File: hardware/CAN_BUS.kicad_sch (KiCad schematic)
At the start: 15 parts, among them U7 ADM3057ExRW

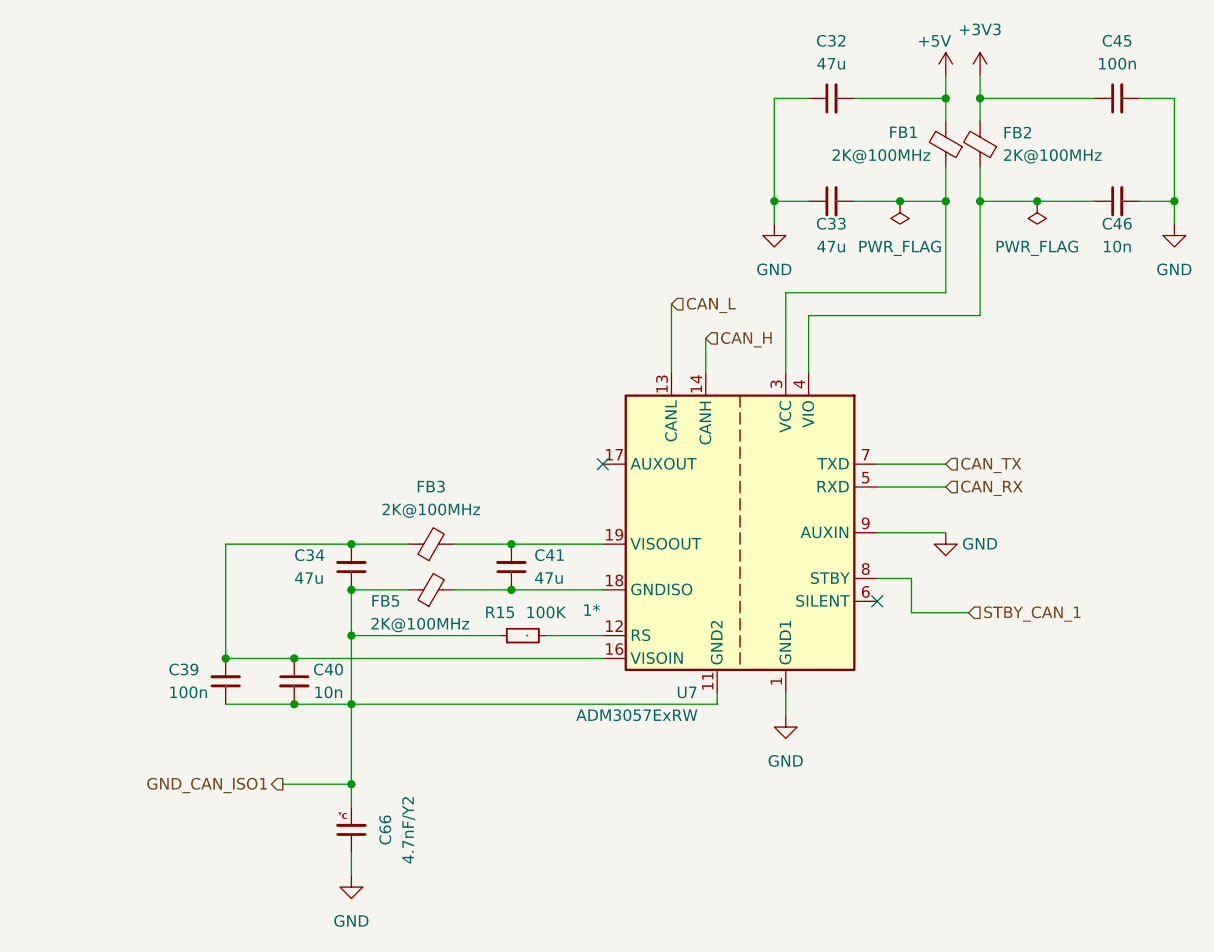
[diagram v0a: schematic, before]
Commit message: added missing files
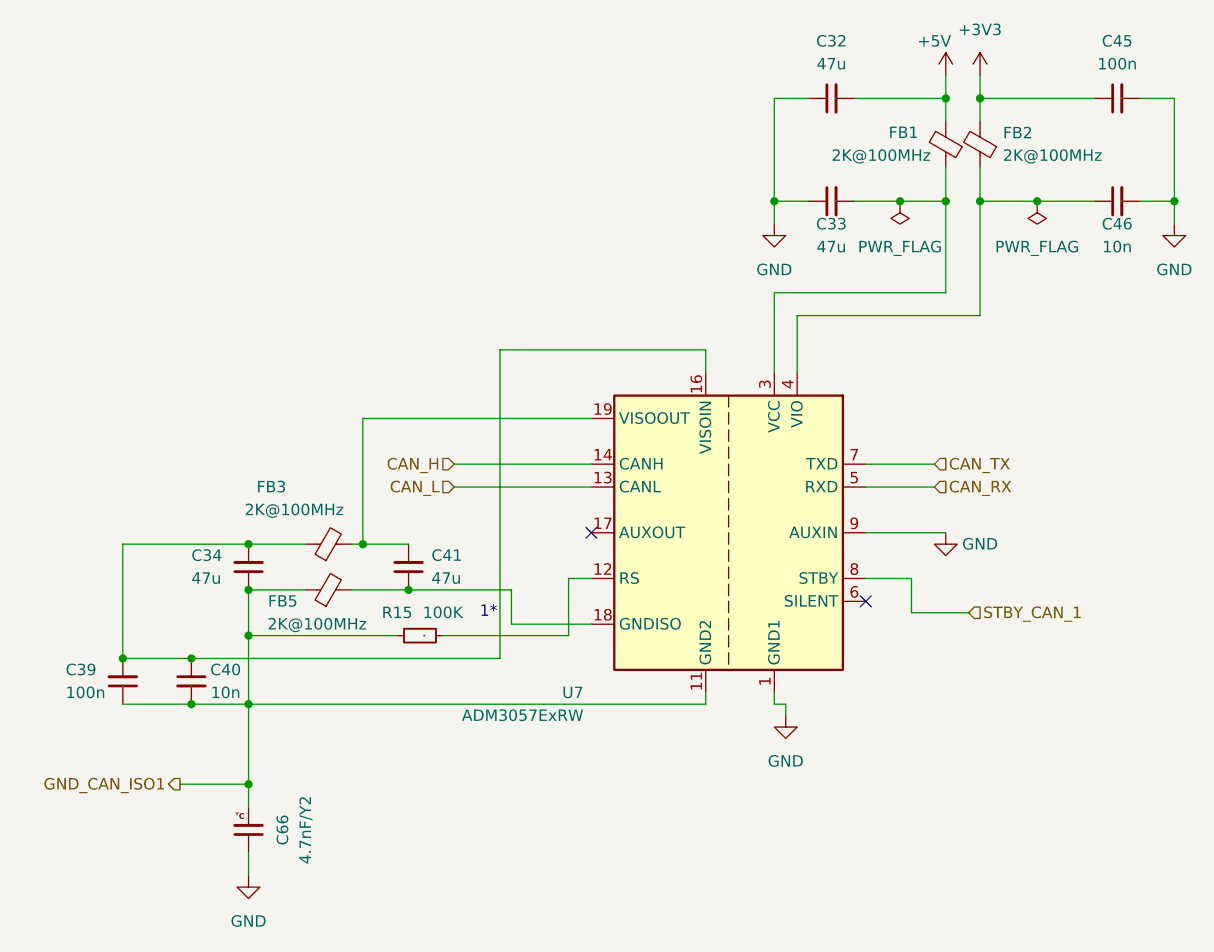
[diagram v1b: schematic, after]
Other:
- moved on the sheet: C34, C39, C40, C41, C66, FB3, FB5, R15, U7
